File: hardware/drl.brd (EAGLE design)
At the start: 56.5 x 32.4 mm, 27 parts, among them IC1 TINY13-20SU, Q1 IRF3205, Q2 IRF3205, T1 BC817-40, X1 CON1, X2 CON2

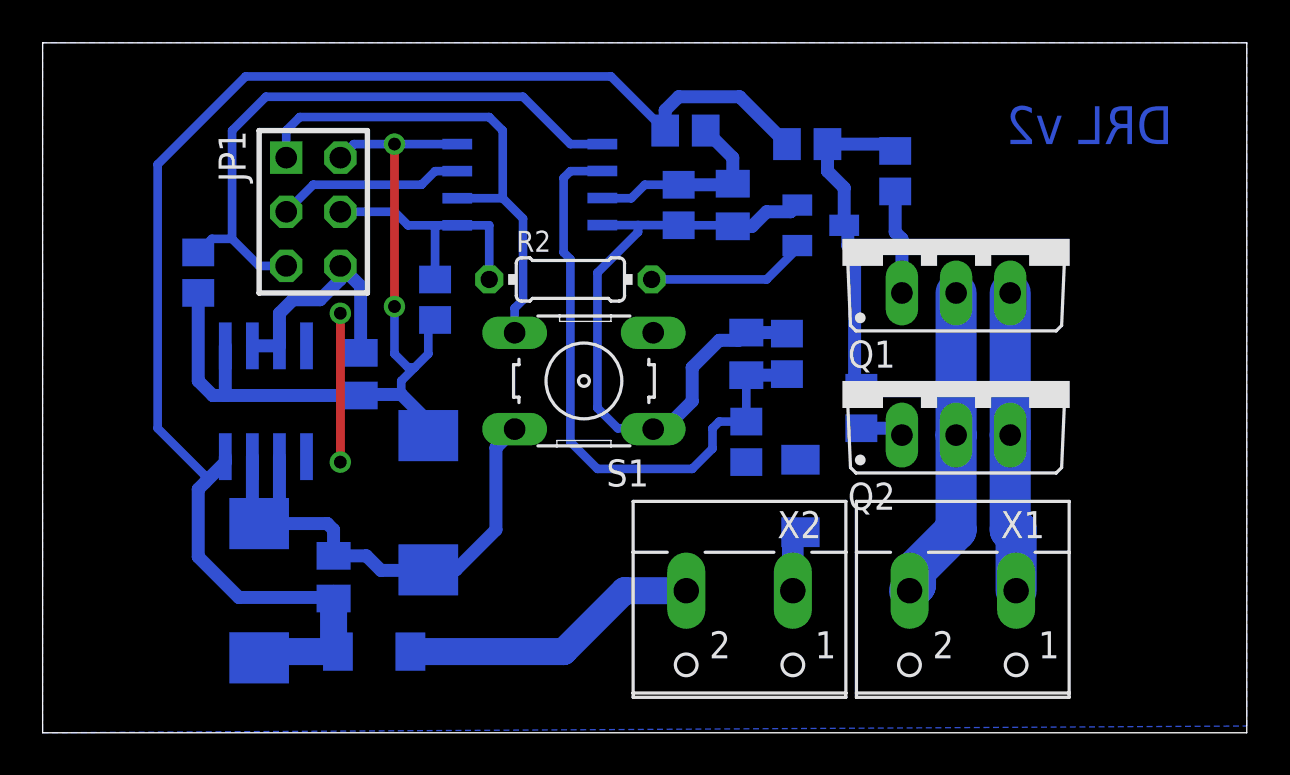
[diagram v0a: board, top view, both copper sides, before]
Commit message: Small editions in schematic and board design.
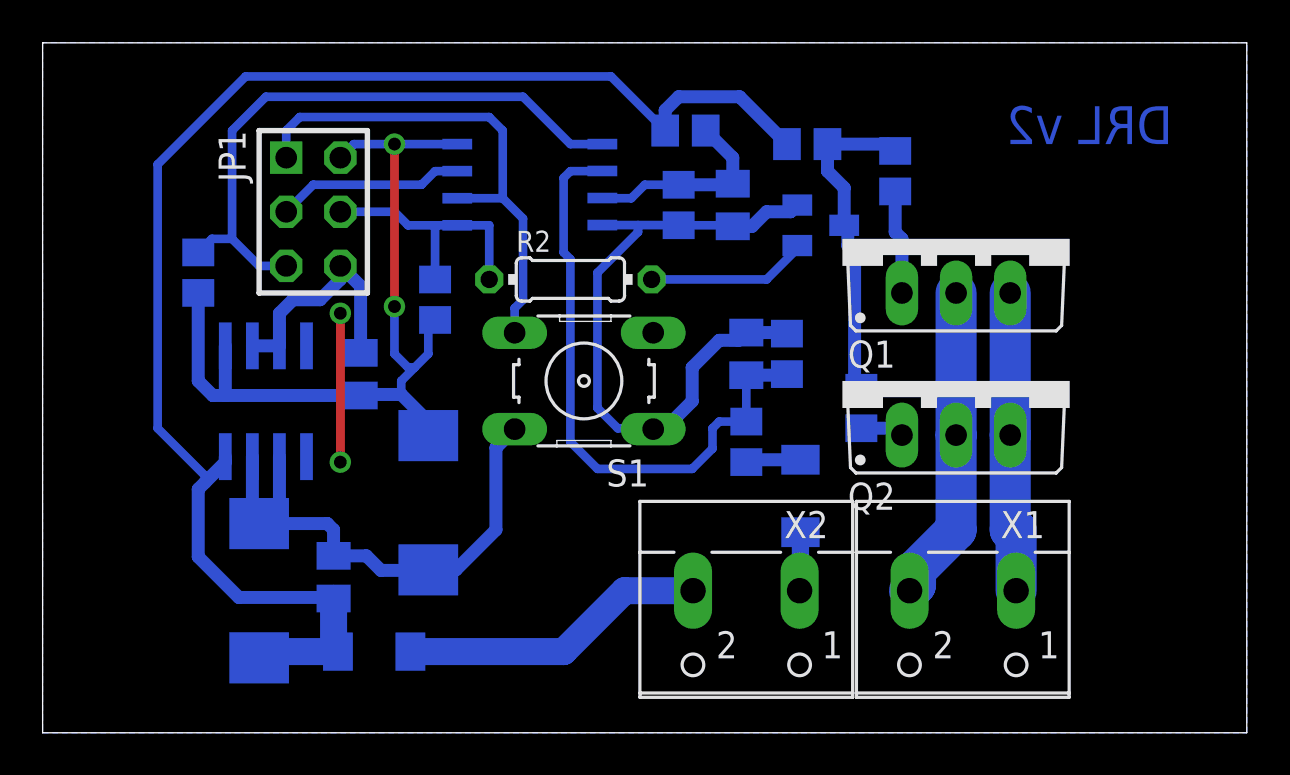
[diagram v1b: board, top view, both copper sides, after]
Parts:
- D1, D2: value (none) -> LL4148
- IC2: value (none) -> 5V
- S1: value (none) -> MODE
- moved X2 0.32 mm to (33.0, 5.40)
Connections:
- net N$7 renamed LOW_BEAM_IN
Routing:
- net N$2: track 0.16 -> 2.81 mm
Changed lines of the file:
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@@
 <attribute name="OC_FARNELL" value="unknown" x="43.18" y="5.3975" size="1.778" layer="27" rot="R180" display="off"/>
 </element>
-<element name="X2" library="con-wago-500" package="W237-102" value="CON2" x="32.7025" y="5.3975" rot="R180">
-<attribute name="OC_NEWARK" value="70K9898" x="32.7025" y="5.3975" size="1.778" layer="27" rot="R180" display="off"/>
-<attribute name="MPN" value="237-102" x="32.7025" y="5.3975" size="1.778" layer="27" rot="R180" display="off"/>
-<attribute name="MF" value="" x="32.7025" y="5.3975" size="1.778" layer="27" rot="R180" display="off"/>
-<attribute name="OC_FARNELL" value="unknown" x="32.7025" y="5.3975" size="1.778" layer="27" rot="R180" display="off"/>
+<element name="X2" library="con-wago-500" package="W237-102" value="CON2" x="33.02" y="5.3975" rot="R180">
+<attribute name="OC_NEWARK" value="70K9898" x="33.02" y="5.3975" size="1.778" layer="27" rot="R180" display="off"/>
+<attribute name="MPN" value="237-102" x="33.02" y="5.3975" size="1.778" layer="27" rot="R180" display="off"/>
+<attribute name="MF" value="" x="33.02" y="5.3975" size="1.778" layer="27" rot="R180" display="off"/>
+<attribute name="OC_FARNELL" value="unknown" x="33.02" y="5.3975" size="1.778" layer="27" rot="R180" display="off"/>
 </element>
 <element name="R2" library="rcl" package="0204/7" value="1k" x="24.765" y="21.2725"/>
-<element name="D1" library="semicon-smd-ipc" package="SOD80" value="" x="15.5575" y="3.81" rot="MR180"/>
+<element name="D1" library="semicon-smd-ipc" package="SOD80" value="LL4148" x="15.5575" y="3.81" rot="MR180"/>
 <element name="R5" library="rcl" package="R0805" value="10k" x="18.415" y="20.32" rot="MR270"/>
 <element name="Q1" library="my_stuff" package="TO220BV" value="IRF3205" x="42.8625" y="23.1775"/>
 <element name="Q2" library="my_stuff" package="TO220BV" value="IRF3205" x="42.8625" y="16.51"/>
-<element name="IC2" library="my_stuff" package="SOIC8" value="" x="10.4775" y="15.5575" rot="MR180"/>
+<element name="IC2" library="my_stuff" package="SOIC8" value="5V" x="10.4775" y="15.5575" rot="MR180"/>
 <element name="C3" library="rcl" package="SMC_D" value="10u" x="10.16" y="6.6675" rot="MR90"/>
 <element name="C4" library="rcl" package="SMC_D" value="10u" x="18.0975" y="10.795" rot="MR270"/>
-<element name="D2" library="semicon-smd-ipc" package="SOD80" value="" x="35.56" y="11.1125" rot="MR270"/>
+<element name="D2" library="semicon-smd-ipc" package="SOD80" value="LL4148" x="35.56" y="11.1125" rot="MR270"/>
 <element name="C5" library="resistor" package="C0805K" value="100n" x="33.02" y="17.78" rot="MR90"/>
 <element name="R8" library="rcl" package="R0805" value="10k" x="29.845" y="24.765" rot="MR270"/>
@@
 <element name="C6" library="resistor" package="C0805K" value="100n" x="32.385" y="24.765" rot="MR270"/>
 <element name="R10" library="rcl" package="R0805" value="10k" x="7.3025" y="21.59" rot="MR90"/>
-<element name="S1" library="switch-omron" package="B3F-10XX" value="" x="25.4" y="16.51" rot="R180">
+<element name="S1" library="switch-omron" package="B3F-10XX" value="MODE" x="25.4" y="16.51" rot="R180">
 <attribute name="OC_NEWARK" value="36M3542" x="25.4" y="16.51" size="1.778" layer="27" rot="R180" display="off"/>
 <attribute name="MPN" value="B3F-1000" x="25.4" y="16.51" size="1.778" layer="27" rot="R180" display="off"/>
@@
 <polygon width="0.4064" layer="16" isolate="0.8128">
 <vertex x="0" y="0"/>
-<vertex x="56.515" y="0.3175"/>
+<vertex x="56.515" y="0"/>
 <vertex x="56.515" y="32.385"/>
 <vertex x="0" y="32.385"/>
@@
 <wire x1="13.97" y1="12.7" x2="13.97" y2="19.685" width="0.4064" layer="1"/>
 <via x="13.97" y="19.685" extent="1-16" drill="0.6"/>
-<wire x1="26.035" y1="15.24" x2="22.1488" y2="14.2494" width="0" layer="19" extent="16-16"/>
+<wire x1="22.1488" y1="14.2494" x2="26.035" y2="15.24" width="0" layer="19" extent="16-16"/>
 </signal>
 <signal name="HI_BEAM">
@@
 <contactref element="D1" pad="2"/>
 <contactref element="X2" pad="2"/>
-<wire x1="30.2025" y1="6.6675" x2="27.305" y2="6.6675" width="1.27" layer="16"/>
+<wire x1="30.52" y1="6.6675" x2="27.305" y2="6.6675" width="1.27" layer="16"/>
 <wire x1="27.305" y1="6.6675" x2="24.4475" y2="3.81" width="1.27" layer="16"/>
 <wire x1="24.4475" y1="3.81" x2="17.2575" y2="3.81" width="1.27" layer="16"/>
@@
 <contactref element="D2" pad="1"/>
 <wire x1="33.02" y1="12.7025" x2="32.91" y2="12.8125" width="0.6096" layer="16"/>
-<wire x1="33.02" y1="12.7025" x2="35.56" y2="12.8125" width="0" layer="19" extent="16-16"/>
+<wire x1="35.56" y1="12.8125" x2="33.02" y2="12.8125" width="0.6096" layer="16"/>
+<wire x1="33.02" y1="12.8125" x2="33.02" y2="12.7025" width="0.6096" layer="16"/>
 </signal>
 <signal name="N$14">
@@
 <wire x1="20.955" y1="23.8125" x2="20.955" y2="21.2725" width="0.4064" layer="16"/>
 </signal>
-<signal name="N$7">
+<signal name="LOW_BEAM_IN">
 <contactref element="D2" pad="2"/>
 <contactref element="X2" pad="1"/>
-<wire x1="35.2025" y1="6.6675" x2="35.2025" y2="9.3725" width="1.016" layer="16"/>
 <wire x1="35.2025" y1="9.3725" x2="35.56" y2="9.4125" width="1.016" layer="16"/>
+<wire x1="35.52" y1="6.6675" x2="35.56" y2="6.6675" width="0.8128" layer="16"/>
+<wire x1="35.56" y1="6.6675" x2="35.56" y2="9.4125" width="0.8128" layer="16"/>
 </signal>
 <signal name="N$12">
